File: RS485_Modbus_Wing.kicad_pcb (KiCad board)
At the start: 2 copper layers, 50.8 x 22.9 mm, 18 parts, among them J1 feather long, J2 feather short, U1 VOS617A, U2 MAX13487E, U3 VOS617A

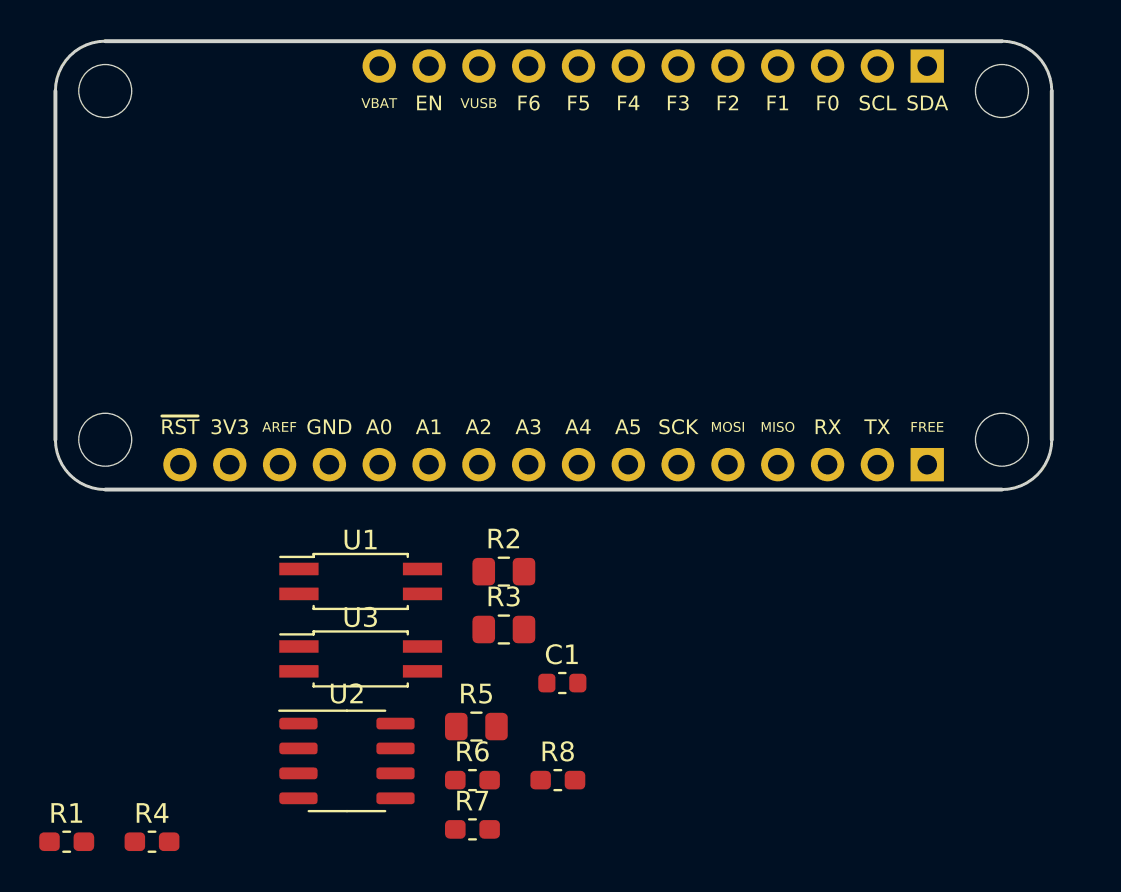
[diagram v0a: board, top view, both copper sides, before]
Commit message: Fist_PCB
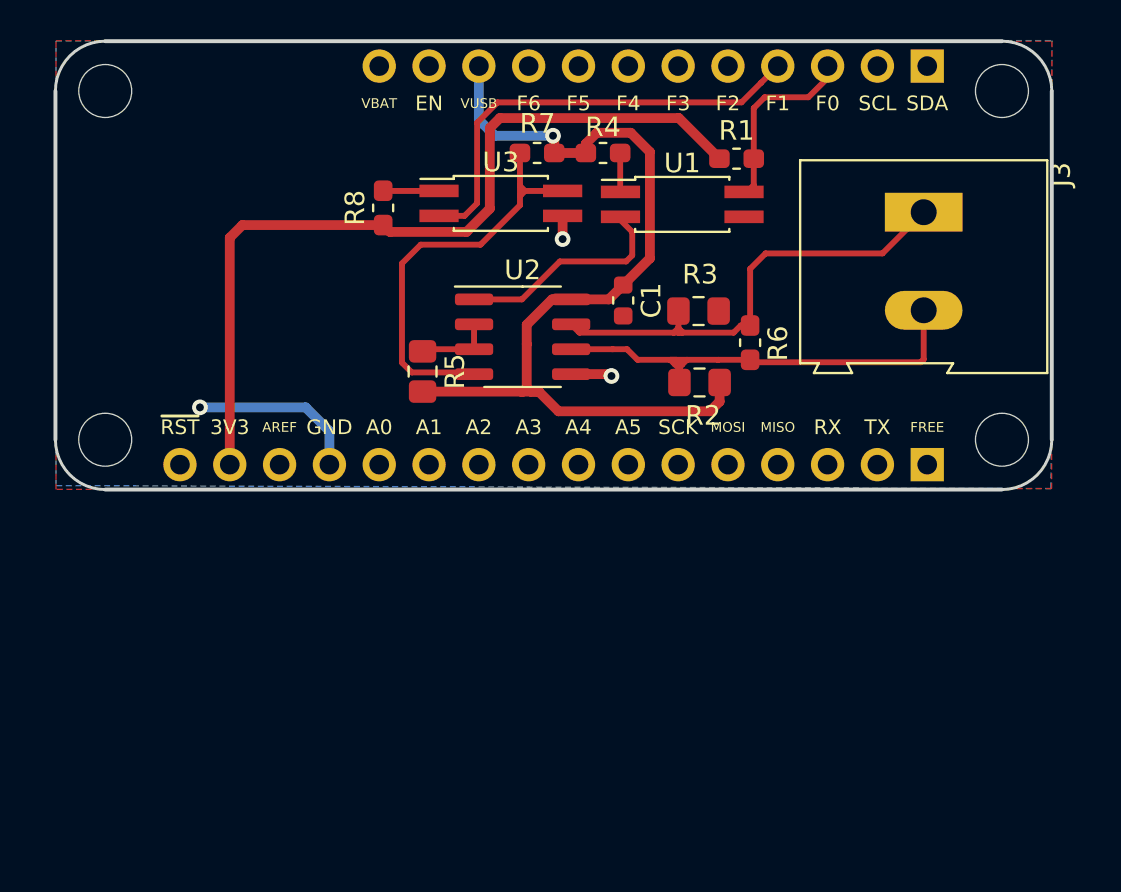
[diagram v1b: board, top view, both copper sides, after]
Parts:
- added J3: Screw_Terminal_01x02, TerminalBlock:TerminalBlock_Altech_AK300-2_P5.00mm, F.Cu at (167.5, 82.9)
- moved R1 48.8 mm to (158.0, 80.2)
- moved R4 42.0 mm to (151.2, 79.9), turned to 180 degrees
- moved R7 34.6 mm to (147.8, 79.9), turned to 180 degrees
- moved R8 30.5 mm to (140.0, 82.7), turned to 90 degrees
- moved R6 26.4 mm to (158.7, 89.5), turned to 90 degrees
- moved U1 25.3 mm to (155.2, 82.5)
- moved U3 24.3 mm to (146.0, 82.4)
- moved U2 23.4 mm to (147.1, 89.2)
- moved C1 19.8 mm to (152.2, 87.4), turned to 270 degrees
- moved R3 19.0 mm to (156.0, 87.9), turned to 180 degrees
- moved R5 18.3 mm to (142.0, 91.0), turned to 270 degrees
- moved R2 13.9 mm to (156.1, 91.6)
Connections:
- J2 pad 10: /VUSB -> VBUS
- J2 pad 3: /D0 -> /D0RX
- J2 pad 4: /D1 -> /D1TX
- R7 pad 2: Net-(R7-Pad2) -> /DI
- U3 pad 4: Net-(R7-Pad2) -> /DI
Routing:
- net VBUS: track 0.00 -> 47.9 mm, vias 0 -> 1
- net +3V3: track 0.00 -> 42.6 mm
- net /B: track 0.00 -> 24.7 mm
- net /A: track 0.00 -> 24.2 mm
- net /D1TX: track 0.00 -> 22.8 mm
- net /DI: track 0.00 -> 21.5 mm
- net GND: track 0.00 -> 12.1 mm, vias 0 -> 3
- net /RO: track 0.00 -> 11.8 mm
- net /D0RX: track 0.00 -> 9.58 mm
- net Net-(R5-Pad1): track 0.00 -> 4.17 mm
- net Net-(R8-Pad2): track 0.00 -> 2.85 mm
- net Net-(R4-Pad1): track 0.00 -> 1.99 mm
- added copper zone on B.Cu, net GND
- added copper zone on F.Cu, net GND
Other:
- net class Default: trace_width 0.25 -> 0.3
- net class Source added: clearance 0.25, trace_width 0.5, via_dia 0.8, via_drill 0.4
